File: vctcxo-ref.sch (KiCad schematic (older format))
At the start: 20 parts, among them IC1 TPS79930, J1 CONN_01x02, J2 CONN_01x02, J3 CONN_01x01, J4 CONN_01x01, J5 CONN_01x01, P1 COAX, P2 COAX, Y1 VCTCXO

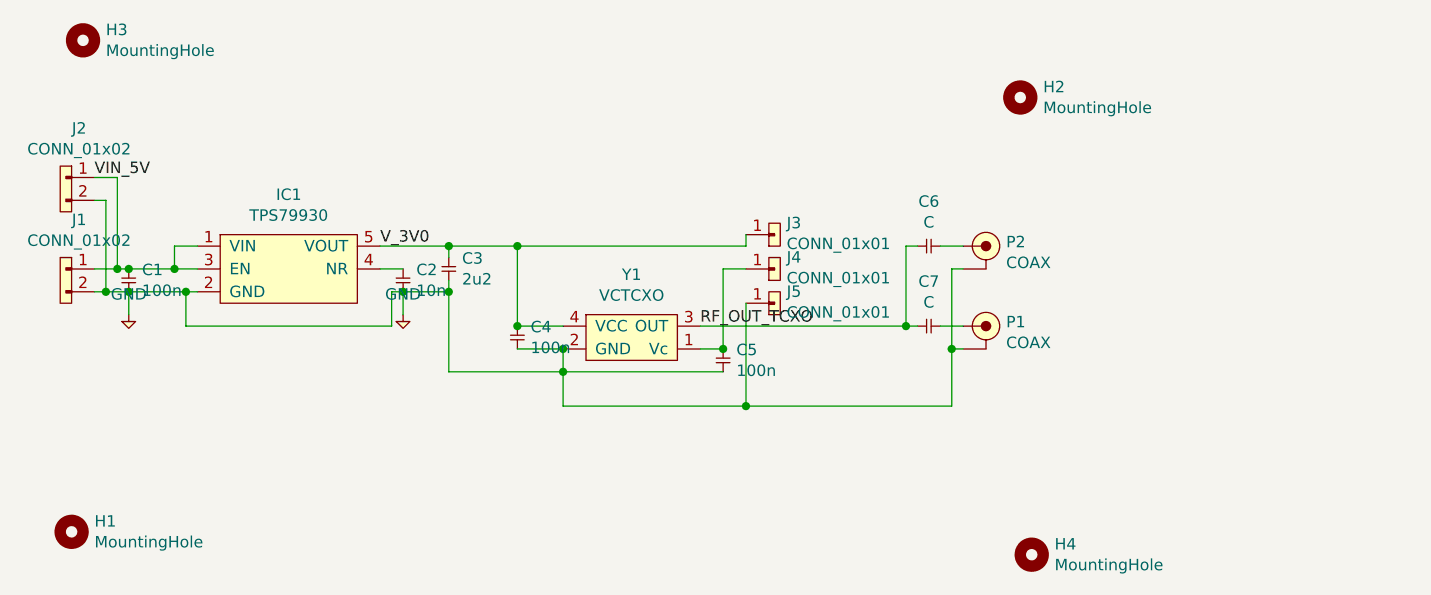
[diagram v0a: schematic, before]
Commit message: Tweaks.
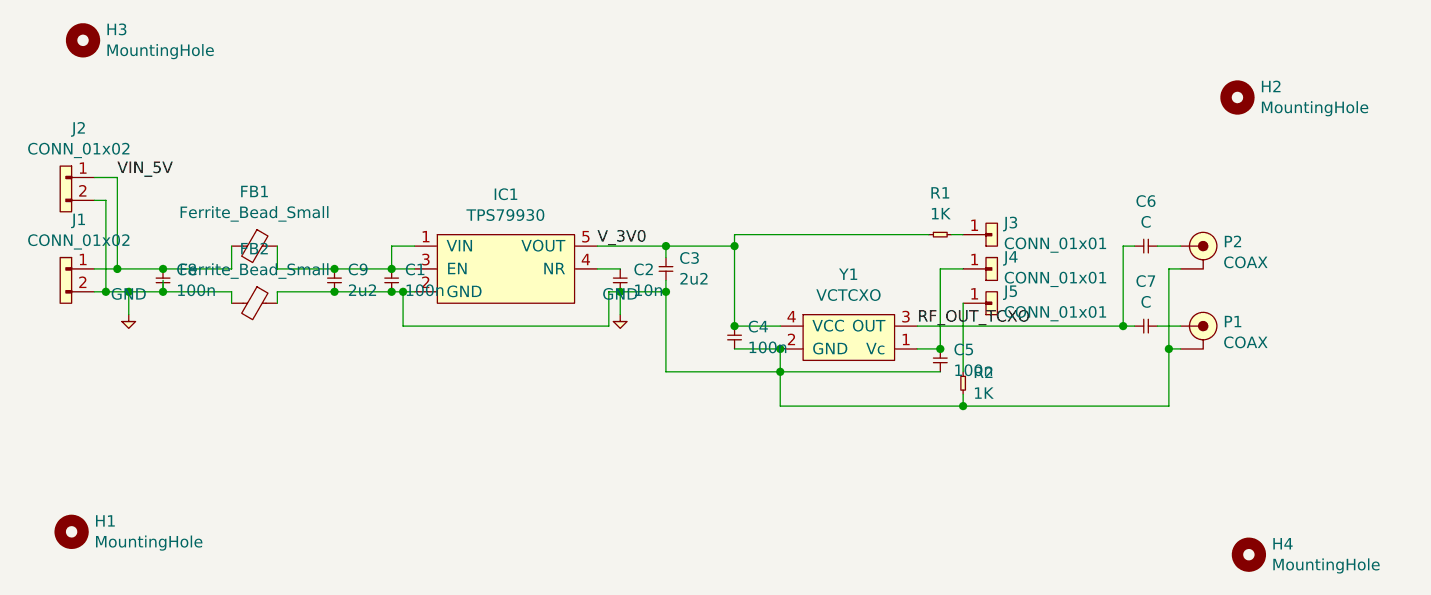
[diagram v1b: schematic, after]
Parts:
- added C8: 100n, agg:0603, symbol agg:C
- added C9: 2u2, agg:0603, symbol agg:C
- added FB1, FB2: Ferrite_Bead_Small, agg:0603, symbol Device:Ferrite_Bead_Small
- added R1, R2: 1K, agg:0603, symbol agg:R
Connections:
- net GND: now also C8.2, C9.1, FB2.1, FB2.2, R2.2; no longer J5.1
- net VIN_5V: now also C8.1, FB1.2; no longer C1.1, IC1.1 (VIN), IC1.3 (EN)
- net V_3V0: now also R1.1; no longer J3.1
- new net: C1.1, C9.2, FB1.1, IC1.1 (VIN), IC1.3 (EN)
- new net: J3.1, R1.2
- new net: J5.1, R2.1
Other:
- moved on the sheet: C1, C2, C3, C4, C5, C6, C7, H2, H4, IC1, J3, J4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

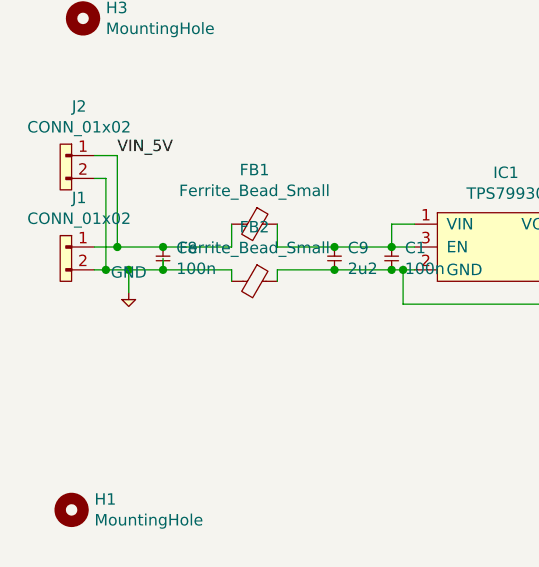
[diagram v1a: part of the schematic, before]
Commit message: Initial plot run.
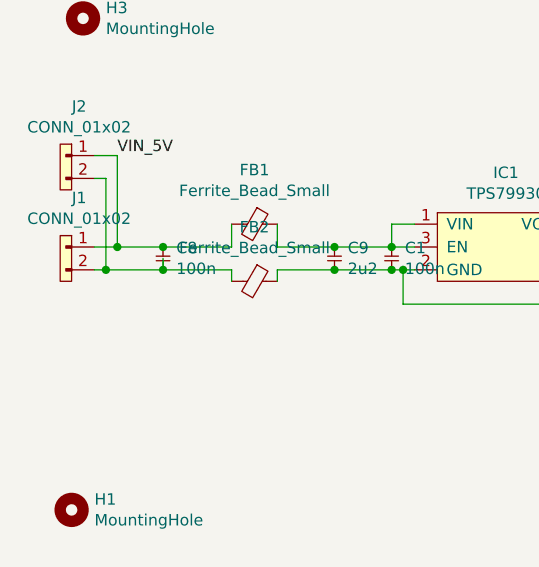
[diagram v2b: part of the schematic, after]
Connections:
- net GND: no longer C8.2, FB2.2, J1.2, J2.2
- new net: C8.2, FB2.2, J1.2, J2.2
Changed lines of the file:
@@
 Wire Wire Line
 	900  2800 950  2800
-$Comp
-L agg:GND #PWR0101
-U 1 1 5CDD7D81
-P 1050 2900
-F 0 "#PWR0101" H 920 2940 50  0001 L CNN
-F 1 "GND" H 1050 2989 50  0000 C CNN
-F 2 "" H 1050 2900 50  0001 C CNN
-F 3 "" H 1050 2900 50  0001 C CNN
-	1    1050 2900
-	1    0    0    -1
-$EndComp
-$Comp
-L agg:GND #PWR0102
-U 1 1 5CDD87F7
-P 3200 2900
-F 0 "#PWR0102" H 3070 2940 50  0001 L CNN
-F 1 "GND" H 3200 2989 50  0000 C CNN
-F 2 "" H 3200 2900 50  0001 C CNN
-F 3 "" H 3200 2900 50  0001 C CNN
-	1    3200 2900
-	1    0    0    -1
-$EndComp
-Wire Wire Line
-	1050 2800 1050 2900
 Wire Wire Line
 	3200 2800 3200 2900
 Wire Wire Line
 	3400 2750 3400 2800
-Wire Wire Line
-	3400 2800 3200 2800
 Connection ~ 3200 2800
 Wire Wire Line
@@
 Connection ~ 950  2800
 Wire Wire Line
-	950  2800 1050 2800
-Wire Wire Line
 	900  2300 1000 2300
 Wire Wire Line
@@
 Wire Wire Line
 	2250 2800 2250 2950
-Wire Wire Line
-	2250 2950 3150 2950
-Wire Wire Line
-	3150 2950 3150 2800
 Wire Wire Line
 	3150 2800 3200 2800
@@
 Connection ~ 1200 2800
 Wire Wire Line
-	1050 2800 1200 2800
-Connection ~ 1050 2800
+	3400 2800 3200 2800
+Wire Wire Line
+	3150 2950 3150 2800
+Wire Wire Line
+	2250 2950 3150 2950
+$Comp
+L agg:GND #PWR0102
+U 1 1 5CDD87F7
+P 3200 2900
+F 0 "#PWR0102" H 3070 2940 50  0001 L CNN
+F 1 "GND" H 3200 2989 50  0000 C CNN
+F 2 "" H 3200 2900 50  0001 C CNN
+F 3 "" H 3200 2900 50  0001 C CNN
+	1    3200 2900
+	1    0    0    -1
+$EndComp
+Wire Wire Line
+	950  2800 1200 2800
 $EndSCHEMATC
